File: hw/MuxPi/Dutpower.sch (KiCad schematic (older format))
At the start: 29 parts, among them P2 XY2500V-D(5.08)-2PIN, P3 XY2500V-D(5.08)-2PIN, Q1 2N7002, U15 MCP6002-E/SN, U16 ICL7660, U4 ACS712ELCTR-05B-T

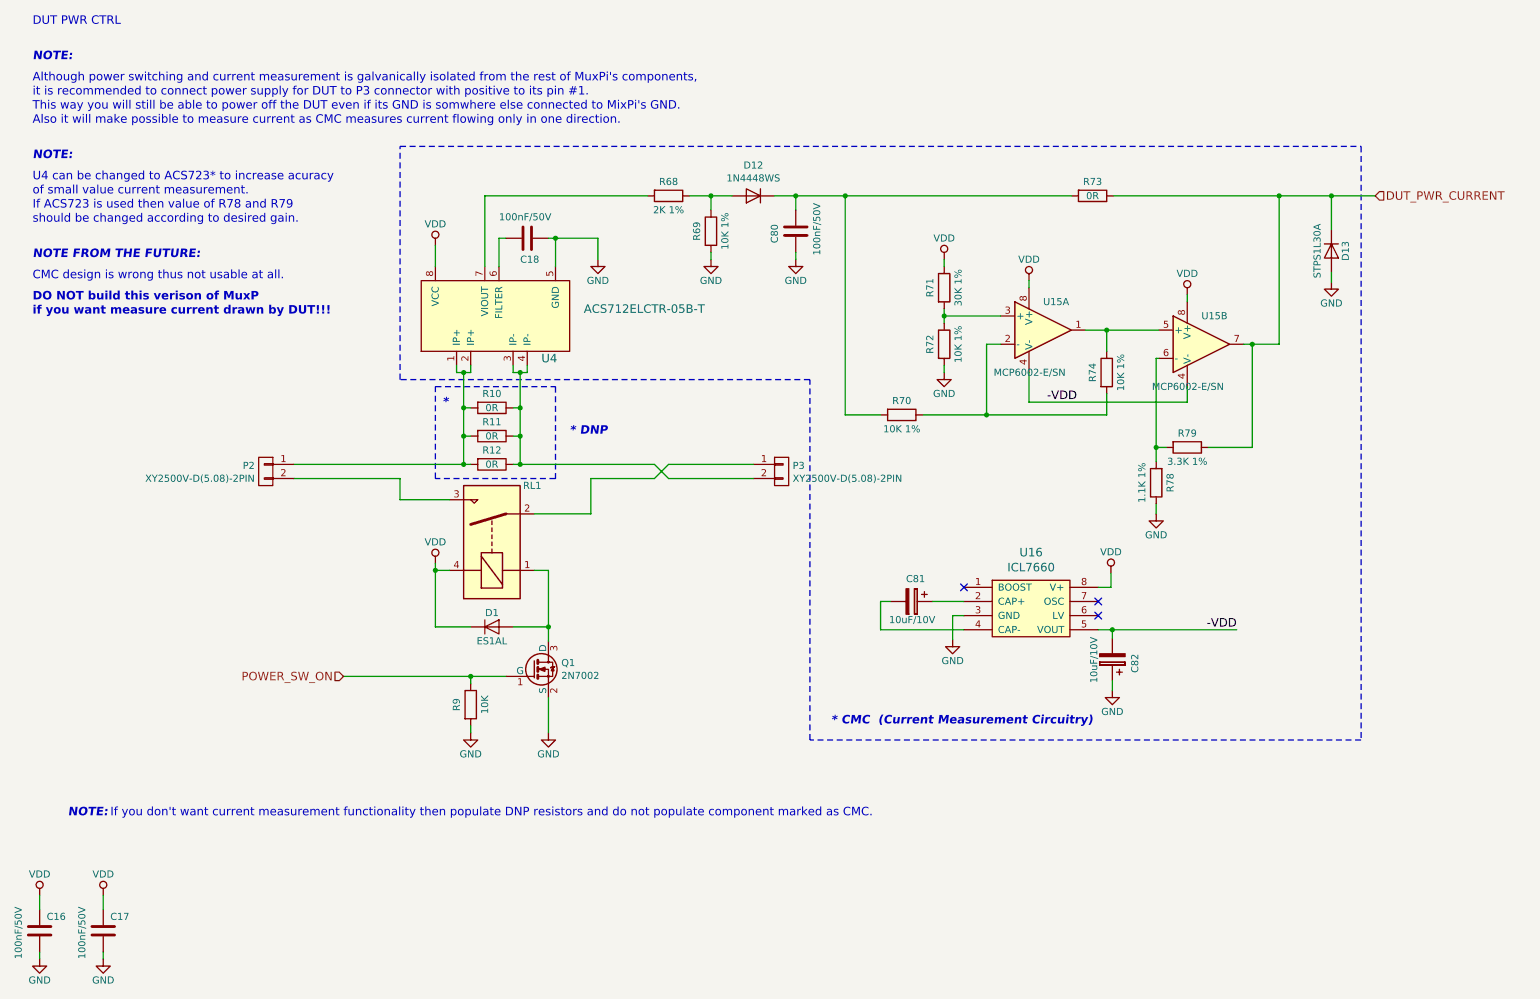
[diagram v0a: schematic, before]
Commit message: Update hardware design to version 1.3
Change-Id: I17b3f32943a6fd048f05d1b0d8676607dc54b976
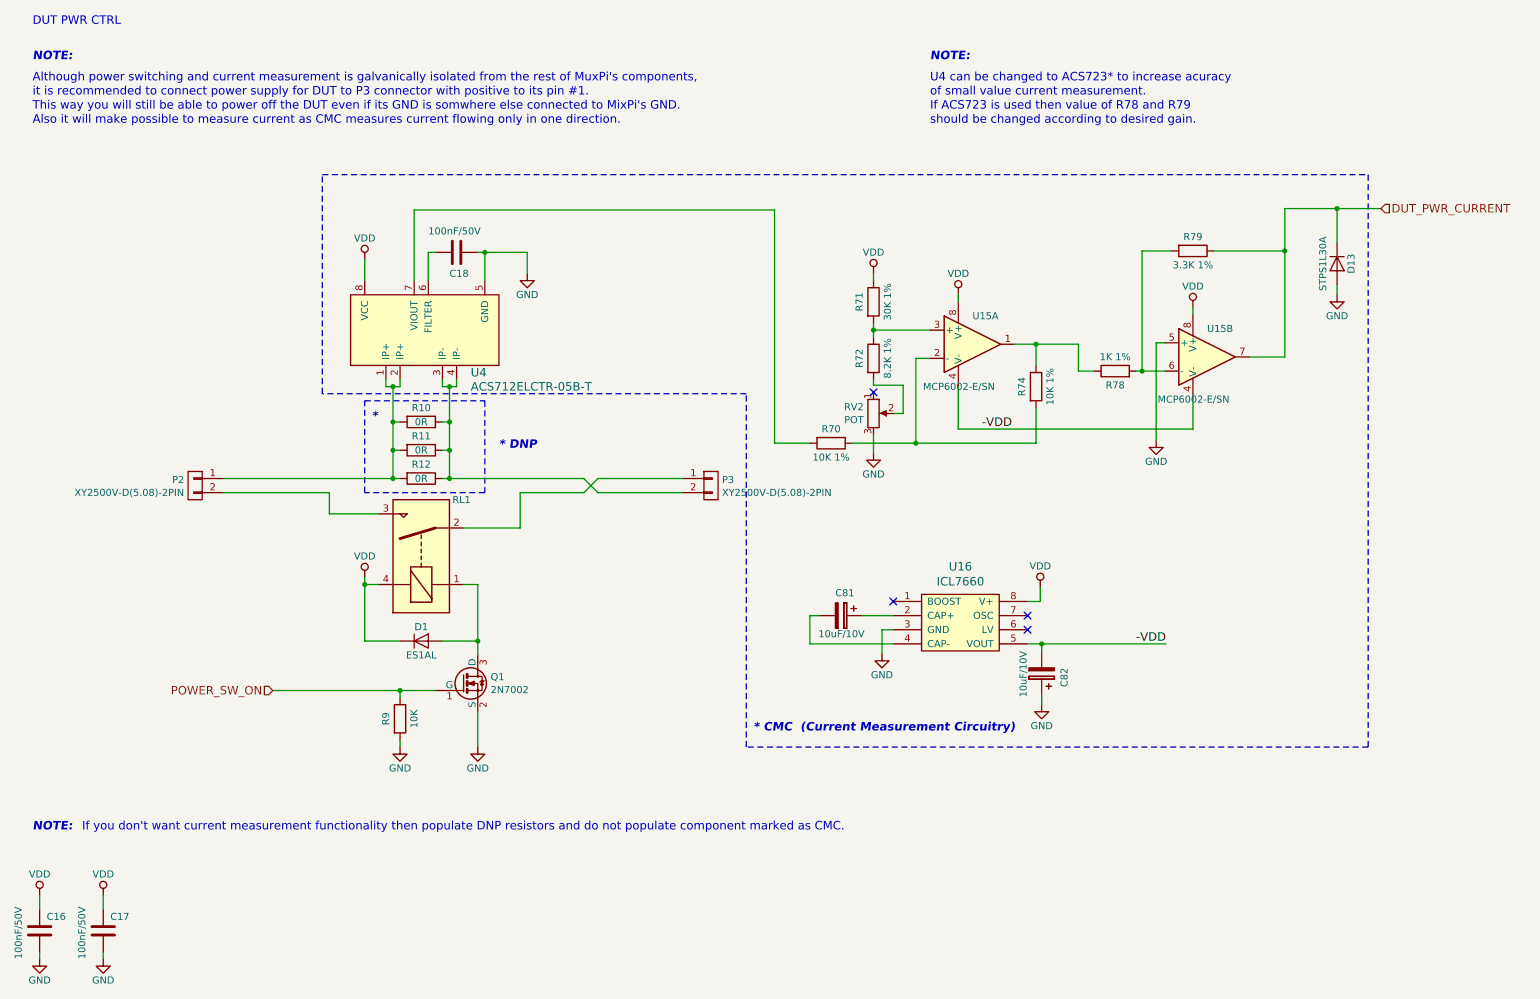
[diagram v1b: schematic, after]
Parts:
- removed C80: 100nF/50V, Capacitors_SMD:C_0805, symbol MuxPi:C
- removed D12: 1N4448WS, Diodes_SMD:D_SOD-323F, symbol MuxPi:D
- removed R68: 2K 1%, Resistors_SMD:R_0805, symbol MuxPi:R
- removed R69: 10K 1%, Resistors_SMD:R_0805, symbol MuxPi:R
- removed R73: 0R, Resistors_SMD:R_0805, symbol MuxPi:R
- added RV2: POT, Potentiometers:Potentiometer_Trimmer_Bourns_3214J, symbol MuxPi:POT
- R72: value 10K 1% -> 8.2K 1%; Shop link http://www.tme.eu/pl/details/rc0805jr-07100k/rezystory-smd-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 -> https://www.tme.eu/pl/details/crcw08058k20fktabc/rezystory-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
- R78: value 1.1K 1% -> 1K 1%
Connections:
- net GND: now also U15.5 (+), RV2.3; no longer R72.2, R78.1
- net at U4.7 (VIOUT): now also R70.2
- net at R74.1, U15.1: now also R78.1; no longer U15.5 (+)
- new net: R72.2, RV2.2
- no-connect marks 3 -> 4
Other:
- note removed: "CMC design is wrong thus not usable at all.\n"
- note removed: "DO NOT build this verison of MuxP"
- note removed: "NOTE FROM THE FUTURE:\n"
- note removed: "if you want measure current drawn by DUT!!!"
- moved on the sheet: C18, C81, C82, D1, D13, P2, P3, Q1, R10, R11, R12, R70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
